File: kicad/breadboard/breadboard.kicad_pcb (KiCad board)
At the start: 2 copper layers, 100 x 100 mm, 22 parts, among them J1 Conn_01x08, J3 Conn_01x08, J4 Conn_01x30, J49 Barrel_Jack, J5 Conn_01x30, J6 Conn_01x30, J7 Conn_01x30, U1 AMS1117-3V3, U2 L7805, U4 bboard_3rows, U5 bboard_3rows

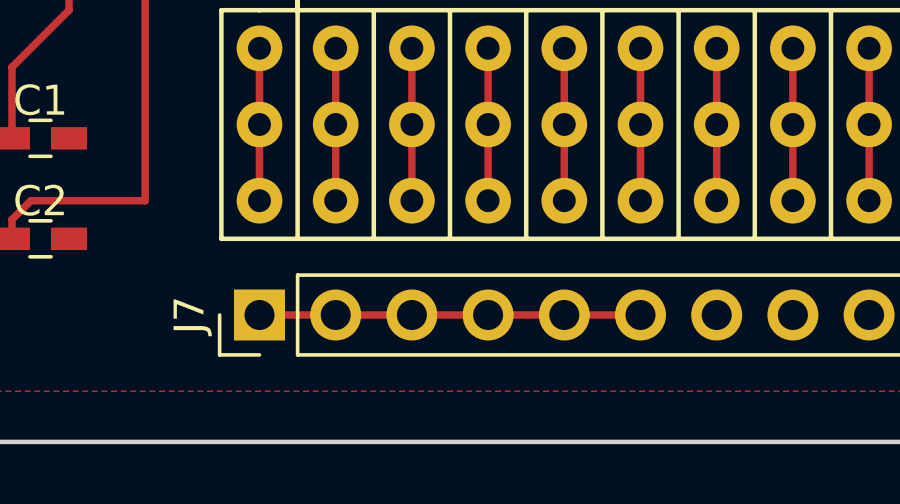
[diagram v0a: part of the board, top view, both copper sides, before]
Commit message: Add gitignore
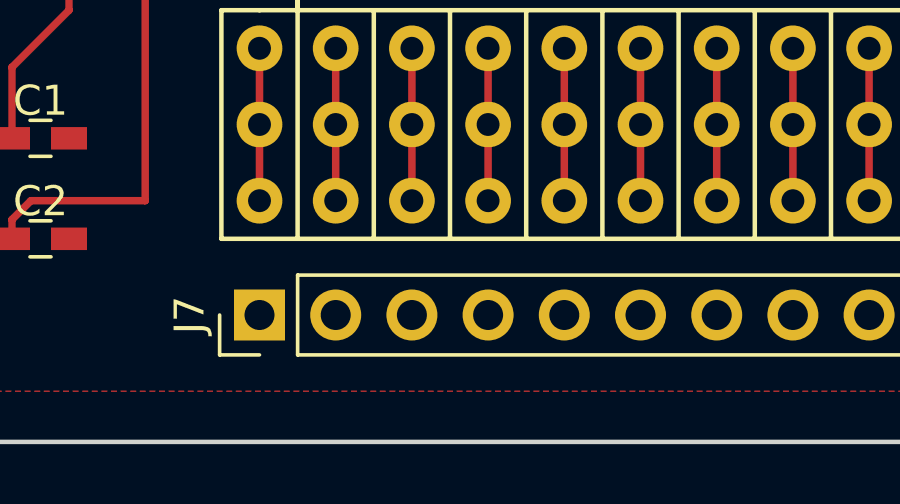
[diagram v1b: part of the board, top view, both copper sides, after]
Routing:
- net GND: track 72.5 -> 59.8 mm
